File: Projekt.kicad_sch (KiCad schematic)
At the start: 115 parts, among them J1 Solar, J2 Battery, J3 USB_B_Mini, J4 INTERFACE PORT, J5 FAN, J6 JTAG, J7 PRG, J8 Micro_SD_Card_Det_Hirose_DM3AT, J9 IIC RTC, Q1 CSD19505KCS, Q11 CSD19505KCS, Q12 CSD19505KCS, Q13 CSD19505KCS, Q2 CSD19505KCS, Q3 CSD19505KCS, Q4 Si2306, Q5 MMBT3904 1A, Q6 MMBT3904 1A, Q7 Si2306, U1 ACS712, U10 ADS1015, U2 B1212S, U3 AMS1117-5.0, U4 AMS1117-3.3, U5 XL7005A, U6 XL7005A, U7 IR2104, U8 ESP32, U9 CH340G

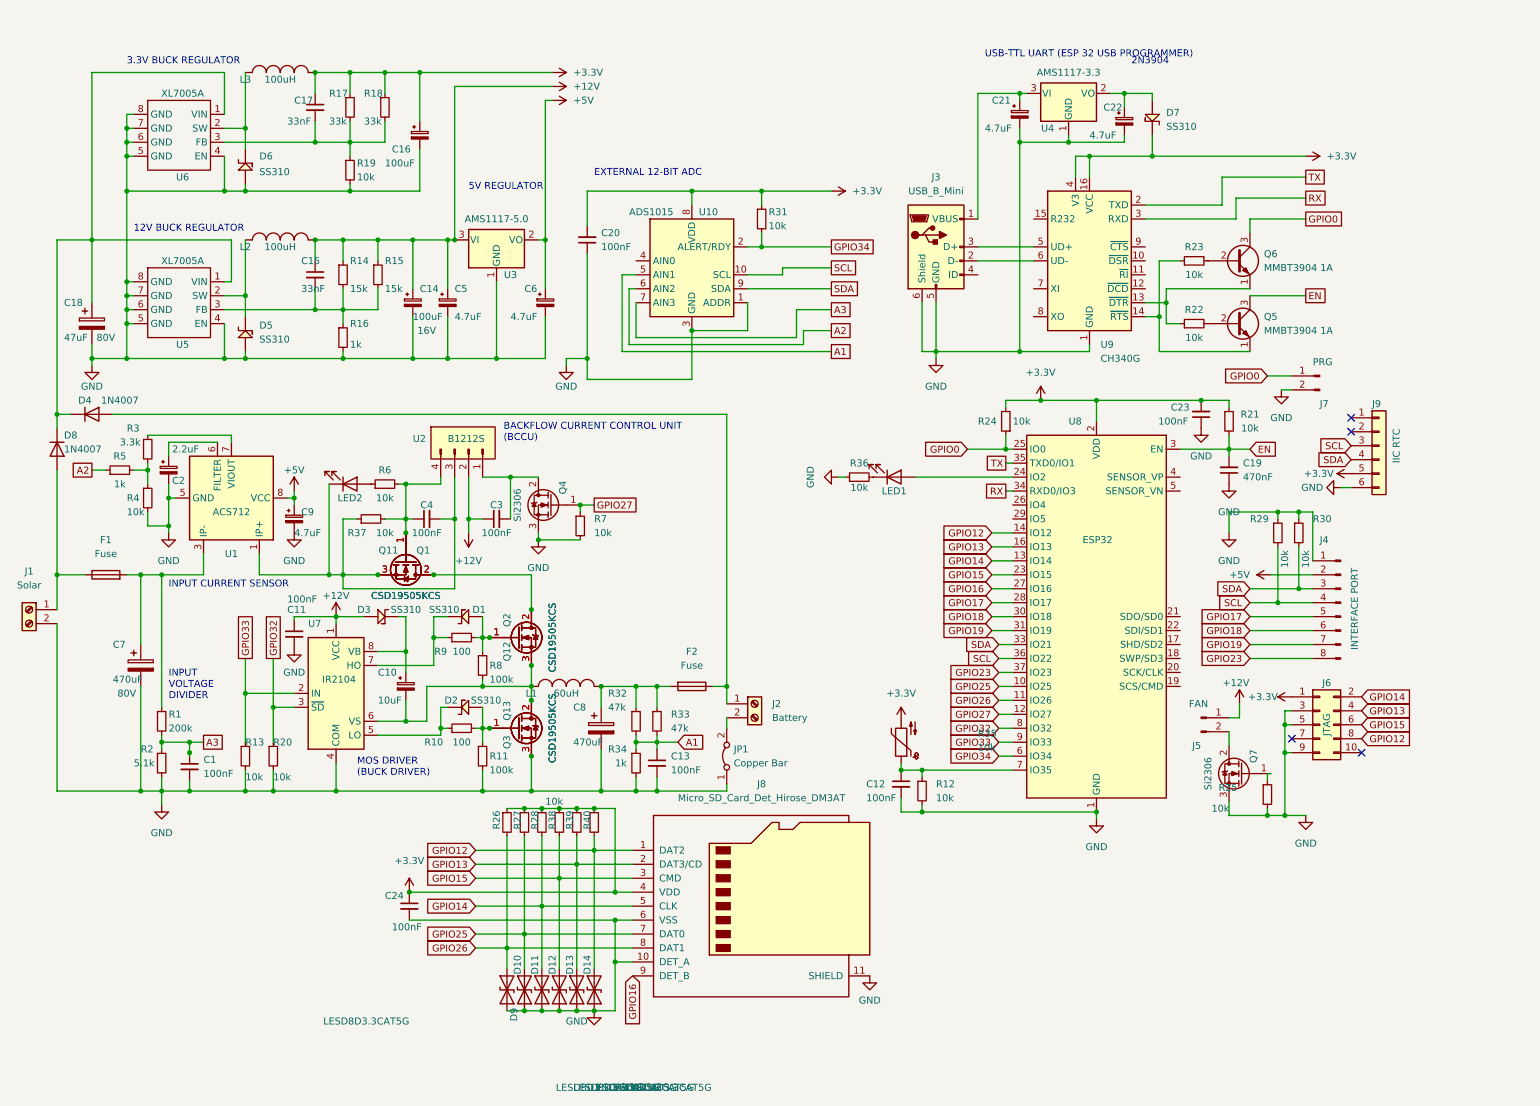
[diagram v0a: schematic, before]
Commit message: Sieht ganz gut aus...
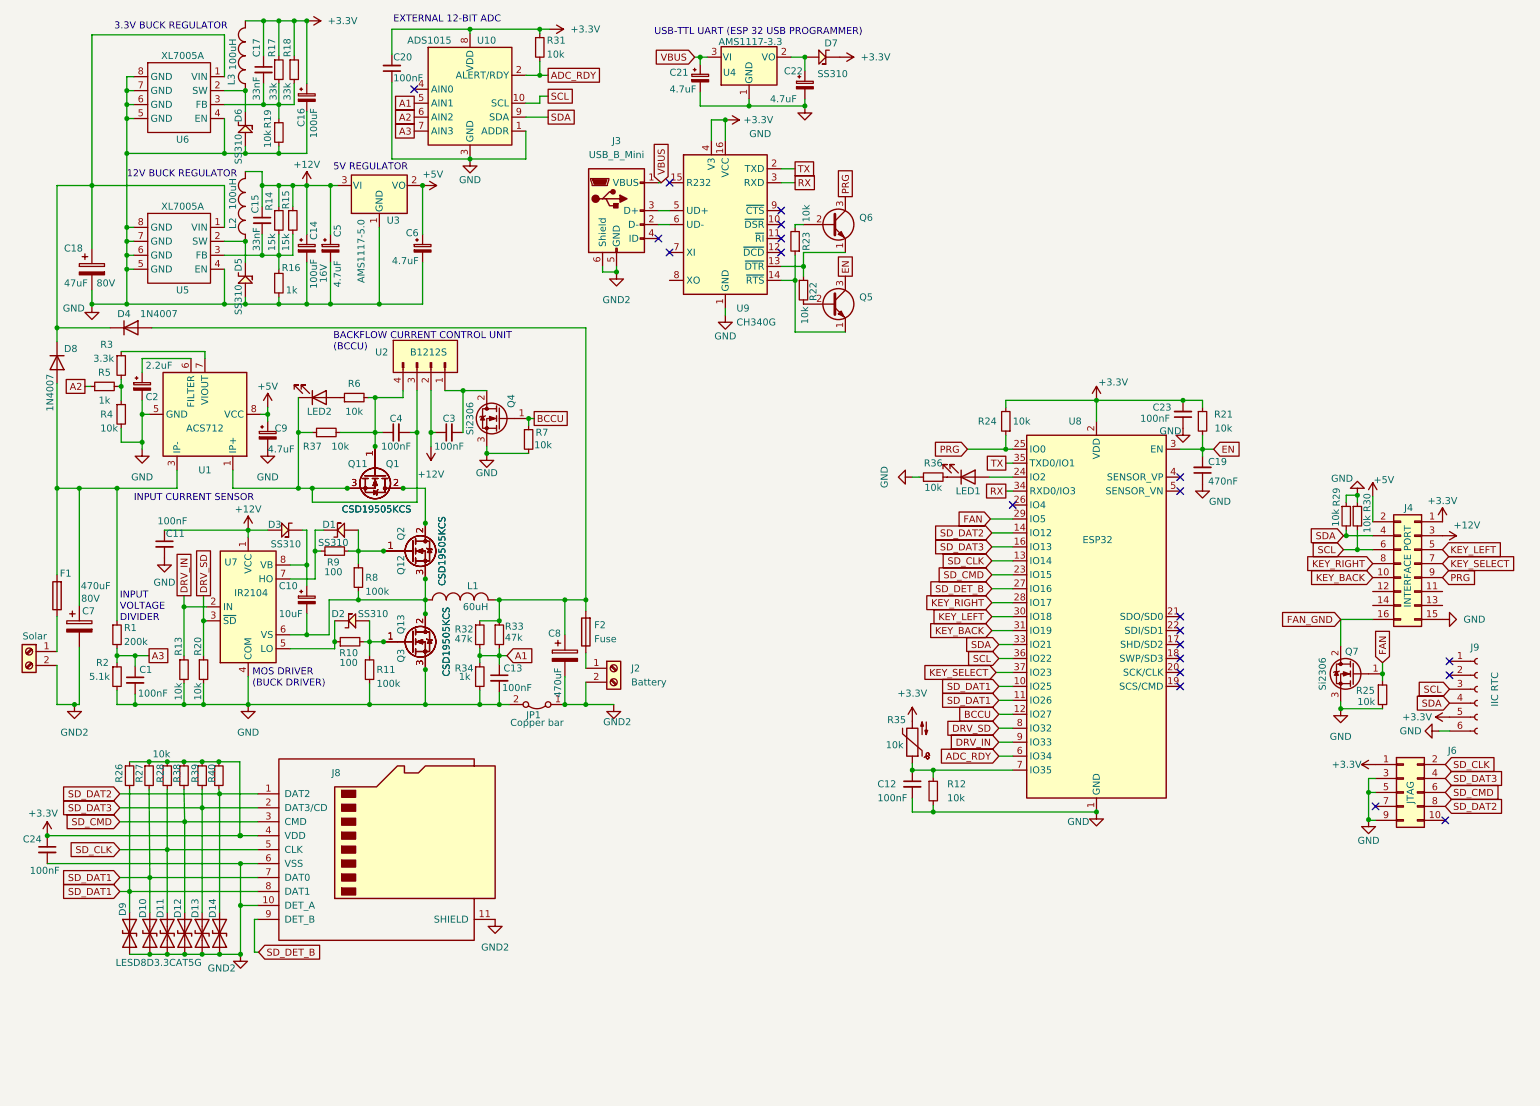
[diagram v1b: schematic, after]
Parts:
- removed J5: FAN, Connector_PinHeader_2.54mm:PinHeader_1x02_P2.54mm_Vertical, symbol Connector:Conn_01x02_Male
- removed J7: PRG, Connector_PinHeader_2.54mm:PinHeader_1x02_P2.54mm_Vertical, symbol Connector:Conn_01x02_Male
- J4: footprint Connector_PinHeader_2.54mm:PinHeader_1x08_P2.54mm_Vertical -> Connector_PinHeader_1.27mm:PinHeader_2x08_P1.27mm_Vertical_SMD; symbol Connector:Conn_01x08_Male -> Connector_Generic:Conn_02x08_Odd_Even
- J9: symbol Connector_Generic:Conn_01x06 -> Connector:Conn_01x06_Female
- JP1: value Copper Bar -> Copper bar
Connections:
- net GPIO26 is gone; now on net SD_DAT1: D9.1 (A1), J8.8 (DAT1), R26.2, U8.11 (IO26)
- net +12V: now also J4.3 (Pin_3)
- net +3.3V: now also J4.1 (Pin_1)
- net GND: now also J4.15 (Pin_15), JP1.2 (B); no longer C24.2, C7.2, C8.2, D10.1 (A1), D11.1 (A1), D12.1 (A1), D13.1 (A1), D14.1 (A1), D9.2 (A2), J1.2 (Pin_2), J3.5 (GND), J3.6 (Shield), J4.1 (Pin_1), J8.10 (DET_A), J8.11 (SHIELD), J8.6 (VSS), JP1.1 (A)
- net SCL: now also J4.6 (Pin_6), R30.2; no longer J4.4 (Pin_4), R29.2
- net SDA: now also J4.4 (Pin_4), R29.2; no longer J4.3 (Pin_3), R30.2
- net at C8.1, F2.2, L1.2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: now also D4.2 (A)
- net FAN_GND: now reaches Q7.2 (D)
- net FAN_GND: now also J4.16 (Pin_16)
- net at C7.1, F1.2, R1.1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: now also D8.2 (A)
- net VBUS: now reaches C21.1, J3.1 (VBUS), U4.3 (VI)
- net at F2.1, J2.1 (Pin_1): no longer D4.2 (A)
- net GND2: now reaches J2.2 (Pin_2)
- net GND2: now also C24.2, C7.2, C8.2, D10.1 (A1), D11.1 (A1), D12.1 (A1), D13.1 (A1), D14.1 (A1), D9.2 (A2), J1.2 (Pin_2), J3.5 (GND), J3.6 (Shield), J8.10 (DET_A), J8.11 (SHIELD), J8.6 (VSS), JP1.1 (A); no longer JP1.2 (B)
- net FAN: now reaches Q7.1 (G), R25.1
- net FAN: now also U8.29 (IO5)
- net at F1.1, J1.1 (Pin_1): no longer D8.2 (A)
- net GPIO0 renamed PRG
- net PRG: now also J4.9 (Pin_9)
- net GPIO12 renamed SD_DAT2
- net GPIO13 renamed SD_DAT3
- net GPIO14 renamed SD_CLK
- net GPIO15 renamed SD_CMD
- net GPIO16 renamed SD_DET_B
- net GPIO17 renamed KEY_LEFT
- net KEY_LEFT: now also U8.30 (IO18); no longer U8.28 (IO17)
- removed net GPIO18: J4.6 (Pin_6), U8.30 (IO18)
- net GPIO19 renamed KEY_BACK
- net KEY_BACK: now also J4.10 (Pin_10); no longer J4.7 (Pin_7)
- net GPIO23 renamed KEY_RIGHT
- net KEY_RIGHT: now also U8.28 (IO17); no longer U8.37 (IO23)
- net GPIO25 renamed SD_DAT1
- net GPIO27 renamed BCCU
- net GPIO32 renamed DRV_SD
- net GPIO33 renamed DRV_IN
- net GPIO34 renamed ADC_RDY
- new net KEY_SELECT: J4.7 (Pin_7), U8.37 (IO23)
- no-connect marks 4 -> 21
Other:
- note removed: "2N3904"
- moved on the sheet: C1, C10, C11, C12, C13, C14, C15, C16, C17, C18, C19, C2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
